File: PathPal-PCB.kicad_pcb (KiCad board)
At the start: 4 copper layers, 34 parts, among them J1 Raspberry_Pi_2_3, J2 Motor, J3 Button1, J4 Button2, J5 Button3, Q1 AO3400A, Q2 AO3400A, Q3 AO3400A, Q4 AO3400A, U1 Gyro, U2 HR, U3 LiDAR

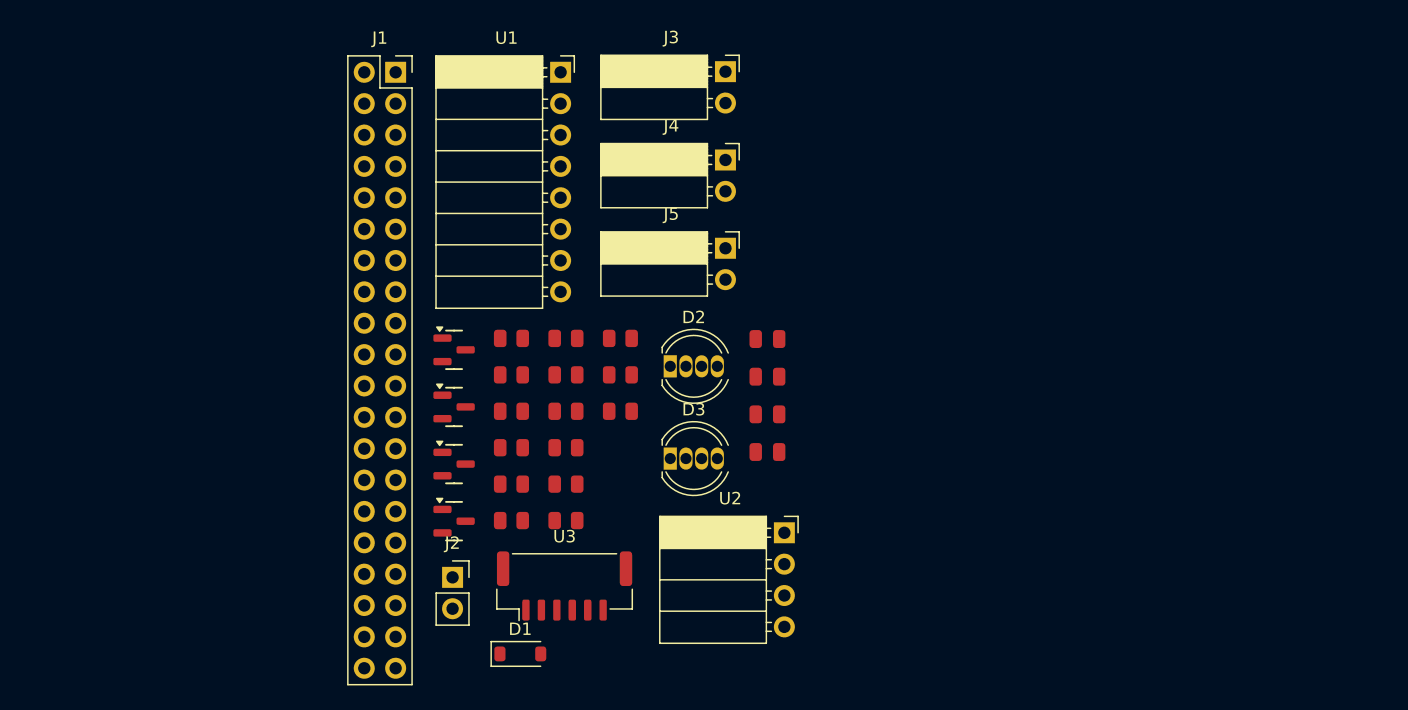
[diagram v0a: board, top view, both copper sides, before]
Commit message: parts layout done
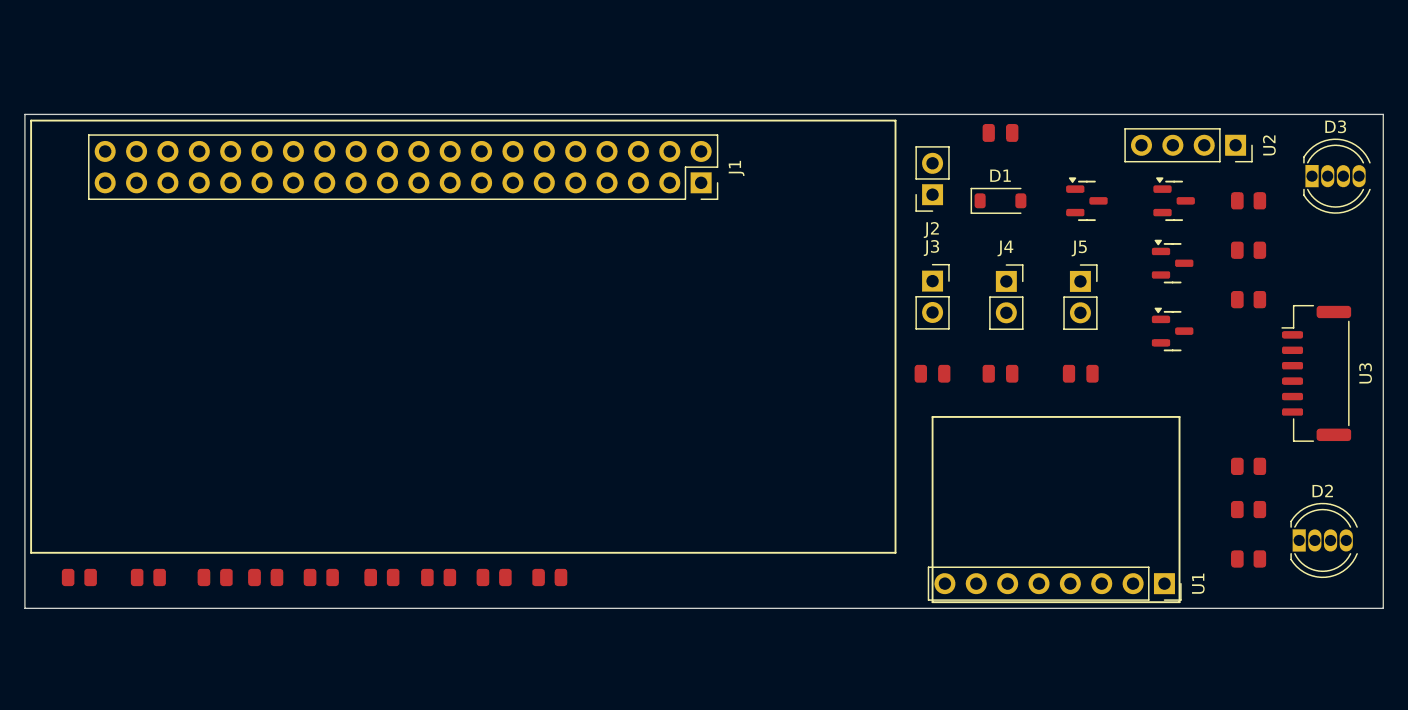
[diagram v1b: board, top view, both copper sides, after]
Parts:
- J3, J4, J5: footprint Connector_PinSocket_2.54mm:PinSocket_1x02_P2.54mm_Horizontal -> Connector_PinSocket_2.54mm:PinSocket_1x02_P2.54mm_Vertical
- U1: footprint Connector_PinSocket_2.54mm:PinSocket_1x08_P2.54mm_Horizontal -> Connector_PinSocket_2.54mm:PinSocket_1x08_P2.54mm_Vertical
- U2: footprint Connector_PinSocket_2.54mm:PinSocket_1x04_P2.54mm_Horizontal -> Connector_PinSocket_2.54mm:PinSocket_1x04_P2.54mm_Vertical
- moved U1 64.1 mm to (177.3, 102.0), turned to -90 degrees
- moved U3 63.3 mm to (189.6, 85.0), turned to -90 degrees
- moved Q2 60.7 mm to (178.1, 71.0)
- moved Q3 60.4 mm to (177.9, 76.0)
- moved Q4 60.2 mm to (177.9, 81.5)
- moved R8 57.0 mm to (184.1, 71.0)
- moved D3 56.8 mm to (189.2, 69.0)
- moved R7 56.2 mm to (184.1, 92.5)
- moved R12 55.4 mm to (184.1, 100.0)
- moved R11 55.3 mm to (184.1, 96.0)
- moved D1 53.5 mm to (164.0, 71.0)
- moved D2 52.8 mm to (188.2, 98.5)
- moved Q1 52.7 mm to (171.0, 71.0)
- moved R13 51.4 mm to (184.1, 75.0)
- moved R14 51.2 mm to (184.1, 79.0)
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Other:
- board outline added: 110 x 40 mm
- rule solder_mask_min_width: 0.12 -> 0.1016

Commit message: moved parts
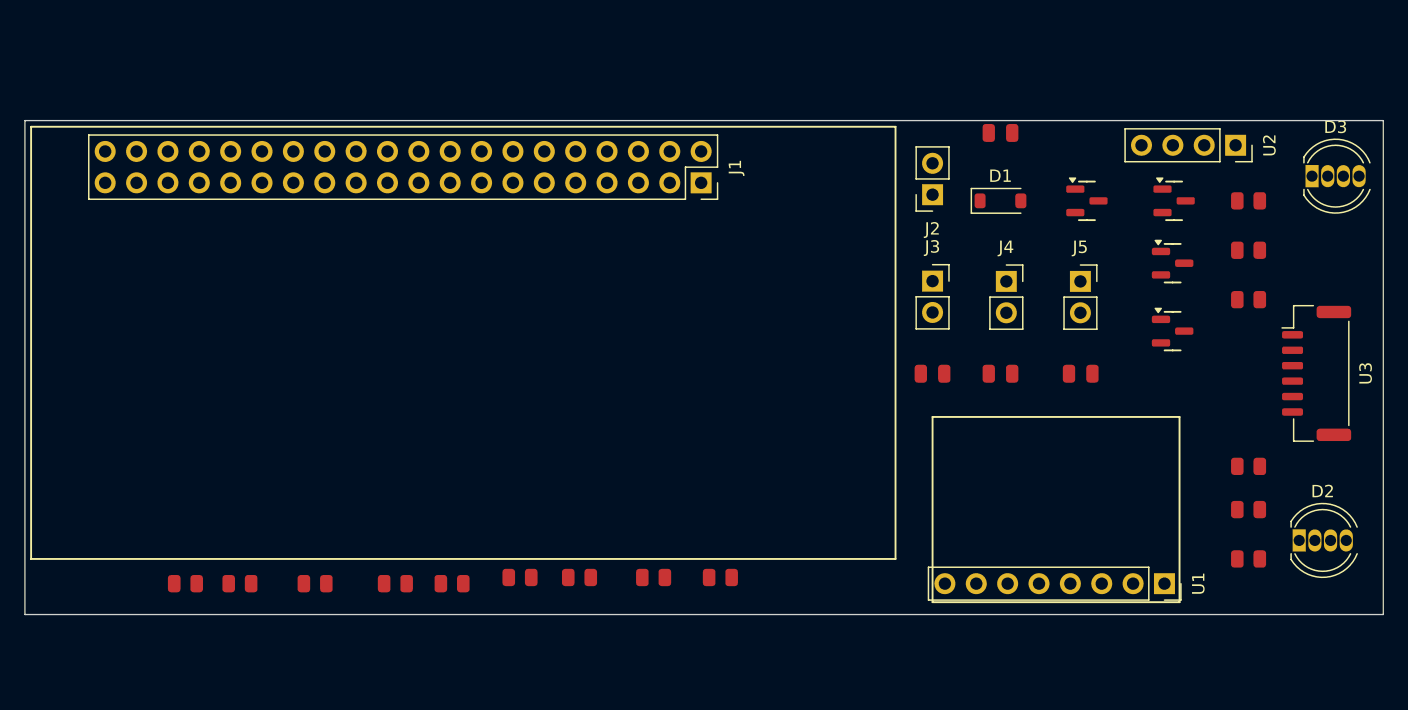
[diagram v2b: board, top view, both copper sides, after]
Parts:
- moved R1 51.9 mm to (141.3, 101.5)
- moved R2 40.9 mm to (135.9, 101.5)
- moved R6 16.1 mm to (125.1, 101.5)
- moved R15 14.5 mm to (108.5, 102.0)
- moved R5 6.52 mm to (98.0, 102.0)
- moved R9 5.70 mm to (119.6, 102.0)
- moved R10 3.54 mm to (115.0, 102.0)
- moved R3 2.41 mm to (129.9, 101.5)
- moved R4 2.06 mm to (102.4, 102.0)
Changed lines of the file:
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@@
 		(13 "F.Paste" user)
 		(15 "B.Paste" user)
-		(5 "F.SilkS" user)
-		(7 "B.SilkS" user)
+		(5 "F.SilkS" user "F.Silkscreen")
+		(7 "B.SilkS" user "B.Silkscreen")
 		(1 "F.Mask" user)
 		(3 "B.Mask" user)
 		(25 "Edge.Cuts" user)
 		(27 "Margin" user)
-		(31 "F.CrtYd" user)
-		(29 "B.CrtYd" user)
+		(31 "F.CrtYd" user "F.Courtyard")
+		(29 "B.CrtYd" user "B.Courtyard")
 		(35 "F.Fab" user)
 	)
@@
 	(footprint "PCM_JLCPCB:R_0805"
 		(layer "F.Cu")
-		(at 109 101.5)
+		(at 125.09 101.5)
 		(descr "Resistor SMD 0805 (2012 Metric), square (rectangular) end terminal, IPC_7351 nominal, (Body size source: IPC-SM-782 page 72, https://www.pcb-3d.com/wordpress/wp-content/uploads/ipc-sm-782a_amendment_1_and_2.pdf), generated with kicad-footprint-generator")
 		(tags "resistor")
@@
 	(footprint "PCM_JLCPCB:R_0805"
 		(layer "F.Cu")
-		(at 89.41 101.5)
+		(at 141.32 101.5)
 		(descr "Resistor SMD 0805 (2012 Metric), square (rectangular) end terminal, IPC_7351 nominal, (Body size source: IPC-SM-782 page 72, https://www.pcb-3d.com/wordpress/wp-content/uploads/ipc-sm-782a_amendment_1_and_2.pdf), generated with kicad-footprint-generator")
 		(tags "resistor")
@@
 	(footprint "PCM_JLCPCB:R_0805"
 		(layer "F.Cu")
-		(at 113.91 101.5)
+		(at 119.59 102)
 		(descr "Resistor SMD 0805 (2012 Metric), square (rectangular) end terminal, IPC_7351 nominal, (Body size source: IPC-SM-782 page 72, https://www.pcb-3d.com/wordpress/wp-content/uploads/ipc-sm-782a_amendment_1_and_2.pdf), generated with kicad-footprint-generator")
 		(tags "resistor")
@@
 	(footprint "PCM_JLCPCB:R_0805"
 		(layer "F.Cu")
-		(at 127.5 101.5)
+		(at 129.91 101.5)
 		(descr "Resistor SMD 0805 (2012 Metric), square (rectangular) end terminal, IPC_7351 nominal, (Body size source: IPC-SM-782 page 72, https://www.pcb-3d.com/wordpress/wp-content/uploads/ipc-sm-782a_amendment_1_and_2.pdf), generated with kicad-footprint-generator")
 		(tags "resistor")
@@
 	(footprint "PCM_JLCPCB:R_0805"
 		(layer "F.Cu")
-		(at 104.5 101.5)
+		(at 98 102)
 		(descr "Resistor SMD 0805 (2012 Metric), square (rectangular) end terminal, IPC_7351 nominal, (Body size source: IPC-SM-782 page 72, https://www.pcb-3d.com/wordpress/wp-content/uploads/ipc-sm-782a_amendment_1_and_2.pdf), generated with kicad-footprint-generator")
 		(tags "resistor")
@@
 	(footprint "PCM_JLCPCB:R_0805"
 		(layer "F.Cu")
-		(at 95 101.5)
+		(at 135.91 101.5)
 		(descr "Resistor SMD 0805 (2012 Metric), square (rectangular) end terminal, IPC_7351 nominal, (Body size source: IPC-SM-782 page 72, https://www.pcb-3d.com/wordpress/wp-content/uploads/ipc-sm-782a_amendment_1_and_2.pdf), generated with kicad-footprint-generator")
 		(tags "resistor")
@@
 	(footprint "PCM_JLCPCB:R_0805"
 		(layer "F.Cu")
-		(at 100.41 101.5)
+		(at 102.41 102)
 		(descr "Resistor SMD 0805 (2012 Metric), square (rectangular) end terminal, IPC_7351 nominal, (Body size source: IPC-SM-782 page 72, https://www.pcb-3d.com/wordpress/wp-content/uploads/ipc-sm-782a_amendment_1_and_2.pdf), generated with kicad-footprint-generator")
 		(tags "resistor")
@@
 	(footprint "PCM_JLCPCB:R_0805"
 		(layer "F.Cu")
-		(at 118.5 101.5)
+		(at 115 102)
 		(descr "Resistor SMD 0805 (2012 Metric), square (rectangular) end terminal, IPC_7351 nominal, (Body size source: IPC-SM-782 page 72, https://www.pcb-3d.com/wordpress/wp-content/uploads/ipc-sm-782a_amendment_1_and_2.pdf), generated with kicad-footprint-generator")
 		(tags "resistor")
@@
 	(footprint "PCM_JLCPCB:R_0805"
 		(layer "F.Cu")
-		(at 123 101.5)
+		(at 108.5 102)
 		(descr "Resistor SMD 0805 (2012 Metric), square (rectangular) end terminal, IPC_7351 nominal, (Body size source: IPC-SM-782 page 72, https://www.pcb-3d.com/wordpress/wp-content/uploads/ipc-sm-782a_amendment_1_and_2.pdf), generated with kicad-footprint-generator")
 		(tags "resistor")
@@
 	)
 	(gr_rect
-		(start 85.5 64.5)
-		(end 155.5 99.5)
+		(start 85.5 65)
+		(end 155.5 100)
 		(stroke
 			(width 0.1524)
@@
 	)
 	(gr_rect
-		(start 85 64)
-		(end 195 104)
+		(start 85 64.5)
+		(end 195 104.5)
 		(stroke
 			(width 0.0381)
